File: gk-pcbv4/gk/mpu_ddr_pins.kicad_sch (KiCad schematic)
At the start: 1 part, among them U5 STM32MP255DAI3

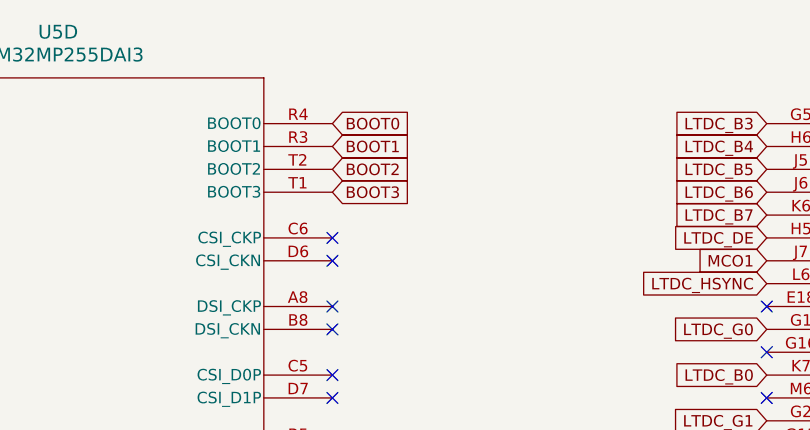
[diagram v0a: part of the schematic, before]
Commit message: pcb order 20251115
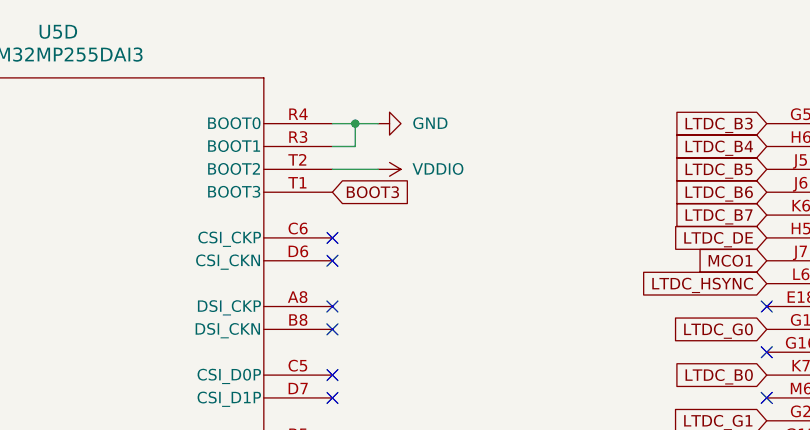
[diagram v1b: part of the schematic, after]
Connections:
- net BOOT1 is gone; now on net GND: U5.R3 (BOOT1)
- net BOOT0 renamed GND
- net BOOT2 renamed VDDIO
